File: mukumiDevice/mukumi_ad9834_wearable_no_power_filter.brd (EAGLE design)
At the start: 54 x 90 mm, 131 parts, among them IC1A1 1k, IC1A1,1 1k, IC1A3'1 560, IC1B1 1k, IC1B2 1k, IC1B6,1 2k, IC2A1,1 5.1k, IC2A3 20k, IC2A3,2 20k, IC2A4 5.1k, IC2B1 20k, IC2B2 5.1k, IC2B3 20k, IC2B6,1 5.1k, IC3A2 56, IC3B1 56, IC4 TL072D, IC4A1 560, IC4A2,2 560, IC4B1 62a, IC4B2 560, IC4B6,1 560a, IC4B6,10 560a, IC4B6,11 560a, IC4B6,12 560a, IC4B6,13 560a, IC4B6,2 560a, IC4B6,3 560a, IC4B6,4 560a, IC4B6,5 560a, IC4B6,6 560a, IC4B6,7 560a, IC4B6,8 560a, IC4B6,9 560a, U1 AD9834, U2 AD9834

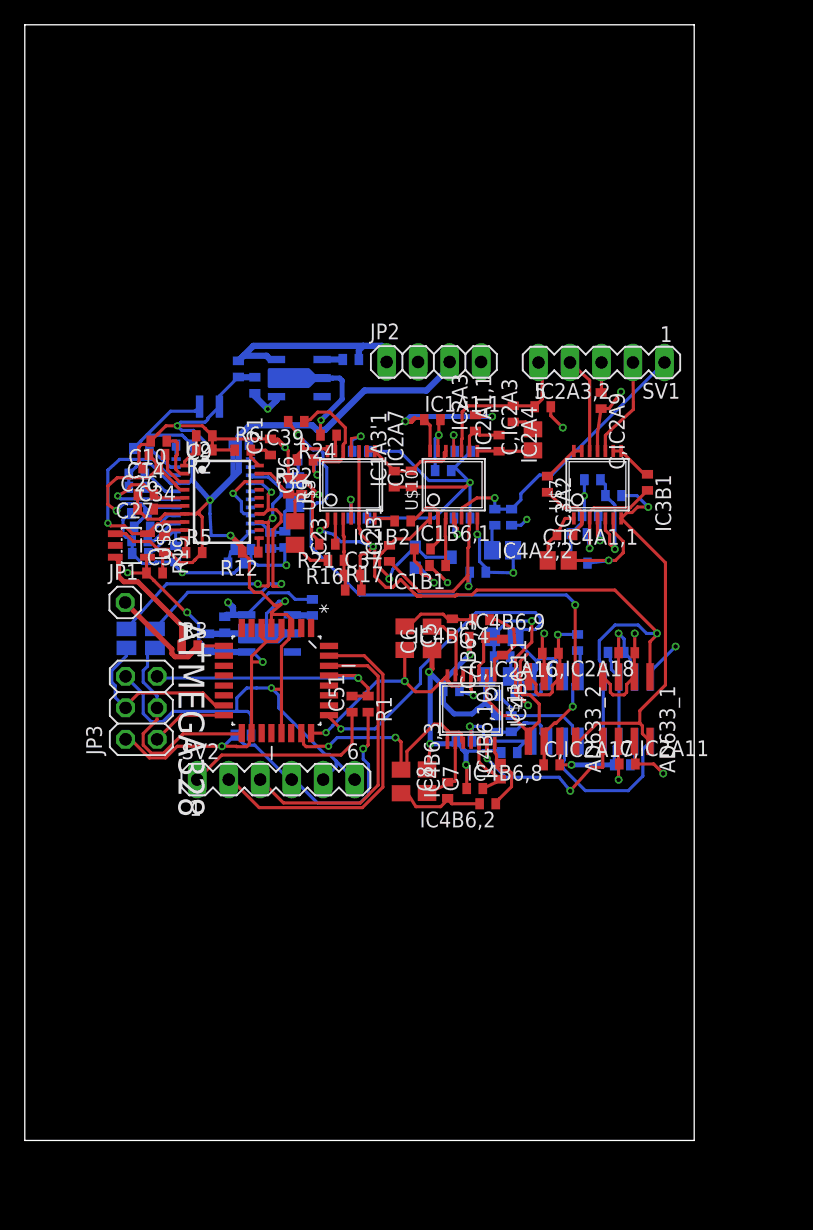
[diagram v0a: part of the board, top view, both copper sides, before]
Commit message: bNAMEの整理と部品名の整理
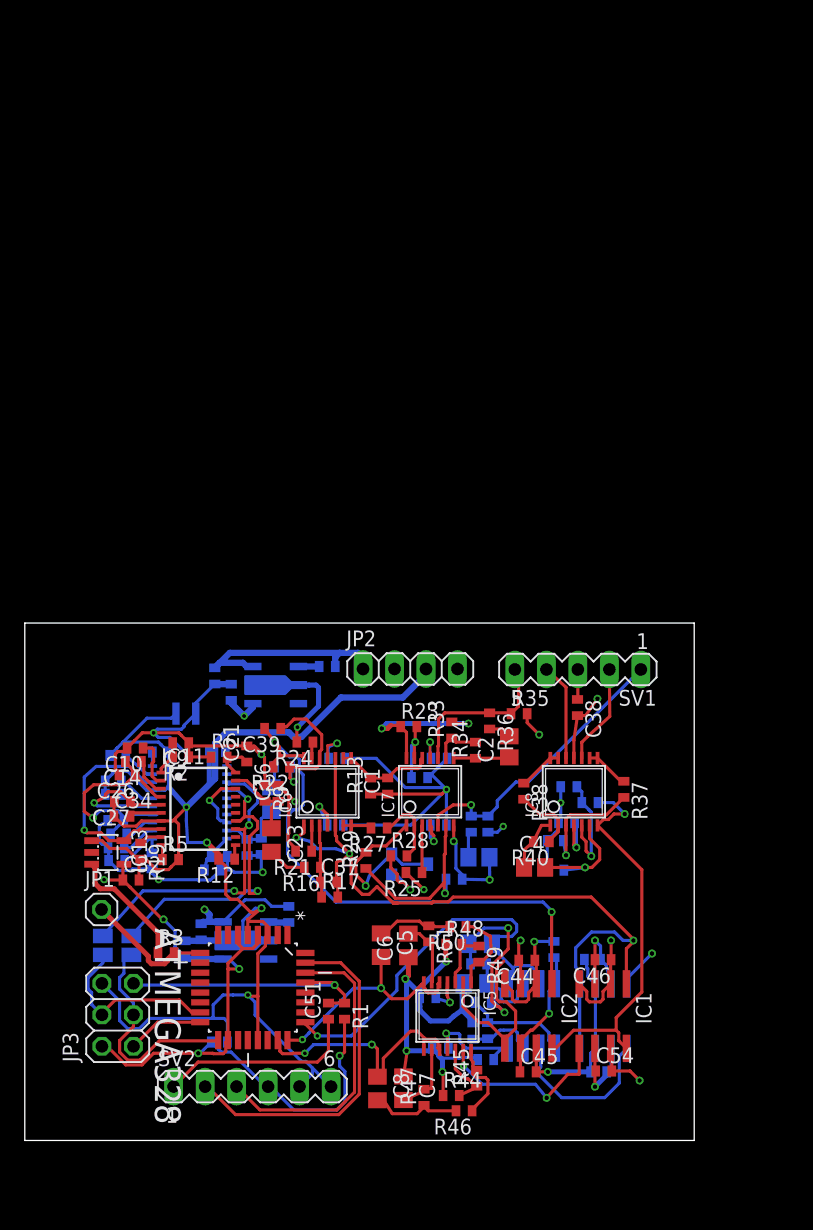
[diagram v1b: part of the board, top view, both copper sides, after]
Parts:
- removed AD633_1, AD633_2, AD633_3: AD835, linear:SO08
- removed C,IC2A1, C,IC2A10, C,IC2A11, C,IC2A12, C,IC2A13, C,IC2A14, C,IC2A15, C,IC2A16, C,IC2A17, C,IC2A18, C,IC2A2, C,IC2A4, C,IC2A5, C,IC2A6, C,IC2A7, C,IC2A8, C,IC2A9: 0.1u, rcl:C0402
- removed C,IC2A3, CIC2B1: 4.7u, rcl:C2012
- removed C,IC4A1,1: 0.47u, rcl:C2012
- removed IC1A1, IC1A1,1, IC1B1, IC1B2: 1k, rcl:R0402
- removed IC1A3'1, IC4A1, IC4A2,2, IC4B2: 560, rcl:R0402
- removed IC1B6,1: 2k, rcl:R0402
- removed IC2A1,1, IC2A4, IC2B2, IC2B6,1: 5.1k, rcl:R0402
- removed IC2A3, IC2A3,2, IC2B1, IC2B3: 20k, rcl:R0402
- removed IC3A2, IC3B1: 56, rcl:R0402
- removed IC4B1: 62a, rcl:R0402
- removed IC4B6,1, IC4B6,10, IC4B6,11, IC4B6,12, IC4B6,13, IC4B6,2, IC4B6,3, IC4B6,4, IC4B6,5, IC4B6,6, IC4B6,7, IC4B6,8, IC4B6,9: 560a, rcl:R0402
- removed L2: CB2016, inductor-yuden:CB2016
- removed U$1, U$2: NJM2884, torex:SOT89-5
- removed U$10, U$11, U$3, U$7: NJM074V, linear:TSSOP14
- removed U$4: PVZ3A, pvz3:PVZ3A
- removed U$8: SIT8002B, memsOsc:SOT25
- removed U1, U2: AD9834, ad9834:TSSOP20
- added C1, C11, C12, C22, C38, C41, C42, C43, C44, C45, C46, C48, C49, C50, C53, C54, C55: 0.1u, rcl:C0402
- added C2, C3: 4.7u, rcl:C2012
- added C4: 0.47u, rcl:C2012
- added IC1, IC2, IC3: AD835, linear:SO08
- added IC10, IC9: NJM2884, torex:SOT89-5
- added IC11, IC12: AD9834, ad9834:TSSOP20
- added IC13: SIT8002B, memsOsc:SOT25
- added IC5, IC6, IC7, IC8: NJM074V, linear:TSSOP14
- added L1: CB2016, inductor-yuden:CB2016
- added R13, R39, R40, R41: 560, rcl:R0402
- added R20, R23, R25, R27: 1k, rcl:R0402
- added R28: 2k, rcl:R0402
- added R29, R32, R33, R35: 20k, rcl:R0402
- added R30, R31, R34, R36: 5.1k, rcl:R0402
- added R37, R38: 56, rcl:R0402
- added R42: 62a, rcl:R0402
- added R43, R44, R45, R46, R47, R48, R49, R50, R51, R52, R53, R54, R55: 560a, rcl:R0402
- added VR1: PVZ3A, pvz3:PVZ3A
- moved C13 24.8 mm to (7.13, 29.0)
- moved C16 24.8 mm to (20.4, 28.0)
- moved C17 24.8 mm to (15.1, 21.8)
- moved C27 24.8 mm to (7.87, 27.3)
- moved C28 24.8 mm to (7.14, 27.9)
- moved C32 24.8 mm to (8.56, 21.0)
- moved C35 24.8 mm to (7.37, 23.6)
- moved C52 24.8 mm to (15.7, 7.93)
- moved R14 24.8 mm to (15.5, 31.4)
- moved R4 24.8 mm to (7.50, 31.1)
- moved ATMEGA328 24.8 mm to (18.4, 12.3)
- moved C18 24.8 mm to (14.2, 16.8)
- moved C19 24.8 mm to (12.9, 15.5)
- moved C20 24.8 mm to (19.1, 23.7)
- moved C23 24.8 mm to (19.9, 24.2)
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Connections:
- net +5V: now also C11.1, C22.1, C41.1, C43.1, C45.1, C48.1, C50.1, C54.1, IC1.6, IC2.6, IC3.6, IC5.4, IC6.4, IC7.4, IC8.4; no longer AD633_1.6, AD633_2.6, AD633_3.6, C,IC2A1.1, C,IC2A11.1, C,IC2A15.1, C,IC2A17.1, C,IC2A2.1, C,IC2A4.1, C,IC2A5.1, C,IC2A6.1, U$10.4, U$11.4, U$3.4, U$7.4
- net +BATTERY: now also IC10.5, IC9.5; no longer U$1.5, U$2.5
- net -5V: now also C12.2, C38.2, C42.2, C44.2, C46.2, C49.2, C53.2, C55.2, IC1.3, IC2.3, IC3.3, IC5.11, IC6.11, IC7.11, IC8.11; no longer AD633_1.3, AD633_2.3, AD633_3.3, C,IC2A10.2, C,IC2A12.2, C,IC2A13.2, C,IC2A14.2, C,IC2A16.2, C,IC2A18.2, C,IC2A8.2, C,IC2A9.2, U$10.11, U$11.11, U$3.11, U$7.11
- net 3.3V_DDS: now also IC10.4, IC11.4, IC12.4; no longer U$2.4, U1.4, U2.4
- net 3.3V_MC: now also IC11.5, IC12.5, IC13.4, IC9.4; no longer U$1.4, U$8.4, U1.5, U2.5
- net A1: now also C3.1, IC7.7, R30.1; no longer CIC2B1.1, IC2B6,1.1, U$10.7
- net AGND: now also C1.1, C11.2, C12.1, C22.2, C38.1, C41.2, C42.1, C43.2, C44.1, C45.2, C46.1, C48.2, C49.1, C50.2, C53.1, C54.2, C55.1, IC1.2, IC1.4, IC1.7, IC10.2, IC11.18, IC12.18, IC2.2, IC2.4, IC2.7, IC3.2, IC3.4, IC3.7, L1.1, R13.1, R20.1, R25.2, R32.2, R35.2, R39.2, R41.1, R42.1, R44.1, R48.1, R52.1; no longer AD633_1.2, AD633_1.4, AD633_1.7, AD633_2.2, AD633_2.4, AD633_2.7, AD633_3.2, AD633_3.4, AD633_3.7, C,IC2A1.2, C,IC2A10.1, C,IC2A11.2, C,IC2A12.1, C,IC2A13.1, C,IC2A14.1, C,IC2A15.2, C,IC2A16.1, C,IC2A17.2, C,IC2A18.1, C,IC2A2.2, C,IC2A4.2, C,IC2A5.2, C,IC2A6.2, C,IC2A7.1, C,IC2A8.1, C,IC2A9.1, IC1A1.1, IC1A3'1.1, IC1B1.2, IC2A3,2.2, IC2B3.2, IC4A1.2, IC4B1.1, IC4B2.1, IC4B6,12.1, IC4B6,8.1, IC4B6,9.1, L2.1, U$2.2, U1.18, U2.18
- net COS: now also IC2.1, IC6.14; no longer AD633_2.1, U$3.14
- net DDS_OUT1: now also IC11.19; no longer U2.19
- net DDS_OUT1B: now also IC11.20; no longer U2.20
- net DDS_OUT2: now also IC12.19; no longer U1.19
- net DDS_OUT2B: now also IC12.20; no longer U1.20
- net DENKYOKU1: now also IC8.12; no longer U$7.12
- net DENKYOKU2: now also IC8.10; no longer U$7.10
- net FSYNC1: now also IC11.15; no longer U2.15
- net FSYNC2: now also IC12.15; no longer U1.15
- net GND: now also IC11.7, IC12.7, IC13.1, IC9.2, L1.2; no longer L2.2, U$1.2, U$8.1, U1.7, U2.7
- net I1: now also IC7.10, R35.1, R36.1; no longer IC2A3,2.1, IC2A4.1, U$10.10
- net I2: now also IC7.5, R31.1, R32.1; no longer IC2B2.1, IC2B3.1, U$10.5
- net N$1: now also IC6.2; no longer U$3.2
- net N$10: now also IC12.6; no longer U1.6
- net N$11: now also IC13.3; no longer U$8.3
- net N$12: now also R53.2, R54.1; no longer IC4B6,13.2, IC4B6,6.1
- net N$13: now also IC9.1; no longer U$1.1
- net N$14: now also IC10.1; no longer U$2.1
- net N$17: now also IC5.12, R44.2, R45.1; no longer IC4B6,10.1, IC4B6,8.2, U$11.12
- net N$19: now also R55.2; no longer IC4B6,7.2
- net N$2: now also IC5.6, R51.2; no longer IC4B6,5.2, U$11.6
- net N$22: now also IC12.1; no longer U1.1
- net N$25: now also IC11.6; no longer U2.6
- net N$26: now also IC7.13, R20.2, R23.2; no longer IC1A1,1.2, IC1A1.2, U$10.13
- net N$27: now also IC11.9; no longer U2.9
- net N$28: now also IC12.9; no longer U1.9
- net N$29: now also IC12.11; no longer U1.11
- net N$3: now also IC5.9, R47.2; no longer IC4B6,3.2, U$11.9
- net N$30: now also IC12.10; no longer U1.10
- net N$33: now also IC7.14, R23.1, R33.2; no longer IC1A1,1.1, IC2A3.2, U$10.14
- net N$38: now also IC12.12; no longer U1.12
- net N$39: now also IC6.13; no longer U$3.13
- net N$4: now also R50.2, R51.1; no longer IC4B6,4.2, IC4B6,5.1
- net N$40: now also IC7.9, R33.1, R34.2; no longer IC2A1,1.2, IC2A3.1, U$10.9
- net N$41: now also C2.2, R36.2; no longer C,IC2A3.2, IC2A4.2
- net N$43: now also IC5.3, R48.2, R49.1; no longer IC4B6,11.1, IC4B6,9.2, U$11.3
- net N$44: now also IC7.6, R29.1, R30.2; no longer IC2B1.1, IC2B6,1.2, U$10.6
- net N$45: now also IC2.5, IC5.2; no longer AD633_2.5, U$11.2
- net N$46: now also C3.2, R31.2; no longer CIC2B1.2, IC2B2.2
- net N$47: now also IC7.2, R27.1, R28.2; no longer IC1B2.1, IC1B6,1.2, U$10.2
- net N$48: now also IC7.1, R29.2, VR1.P$1, VR1.P$3; no longer IC2B1.2, U$10.1, U$4.P$1, U$4.P$3
- net N$49: now also R28.1, VR1.P$2; no longer IC1B6,1.1, U$4.P$2
- net N$5: now also IC1.5, IC5.13; no longer AD633_1.5, U$11.13
- net N$50: now also IC8.13, IC8.14, R38.1; no longer IC3A2.1, U$7.13, U$7.14
- net N$51: now also IC8.8, IC8.9, R37.1; no longer IC3B1.1, U$7.8, U$7.9
- net N$52: now also IC8.3, R37.2, R39.1; no longer IC3B1.2, IC4A1.1, U$7.3
- net N$53: now also IC8.2, R38.2, R40.1; no longer IC3A2.2, IC4A2,2.1, U$7.2
- net N$54: now also C4.1, IC8.1, R40.2; no longer C,IC4A1,1.1, IC4A2,2.2, U$7.1
- net N$55: now also C4.2, IC8.6, R41.2; no longer C,IC4A1,1.2, IC4B2.2, U$7.6
- net N$56: now also C2.1, IC7.8, R34.1; no longer C,IC2A3.1, IC2A1,1.1, U$10.8
- net N$57: now also IC7.3, R25.1; no longer IC1B1.1, U$10.3
- net N$58: now also IC8.5, R42.2, R43.1; no longer IC4B1.2, IC4B6,1.1, U$7.5
- net N$59: now also IC5.14, R45.2, R46.1; no longer IC4B6,10.2, IC4B6,2.1, U$11.14
- net N$6: now also R46.2, R47.1; no longer IC4B6,2.2, IC4B6,3.1
- net N$60: now also IC5.1, R49.2, R50.1; no longer IC4B6,11.2, IC4B6,4.1, U$11.1
- net N$61: now also C1.2, IC6.8, IC6.9, IC7.12, R13.2; no longer C,IC2A7.2, IC1A3'1.2, U$10.12, U$3.8, U$3.9
- net N$62: now also IC6.6, IC6.7, R27.2; no longer IC1B2.2, U$3.6, U$3.7
- net N$63: now also R54.2, R55.1; no longer IC4B6,6.2, IC4B6,7.1
- net N$66: now also IC11.11; no longer U2.11
- net N$67: now also IC11.1; no longer U2.1
- net N$68: now also IC3.5; no longer AD633_3.5
- net N$70: now also R52.2, R53.1; no longer IC4B6,12.2, IC4B6,13.1
- net N$74: now also IC11.10; no longer U2.10
- net N$75: now also IC12.2; no longer U1.2
- net N$77: now also IC12.3; no longer U1.3
- net N$78: now also IC6.3; no longer U$3.3
- net N$79: now also IC11.3; no longer U2.3
- net N$8: now also IC11.8, IC12.8, IC13.5; no longer U$8.5, U1.8, U2.8
- net N$9: now also IC11.2; no longer U2.2
- net N$91: now also IC6.12; no longer U$3.12
- net SCLK: now also IC11.14, IC12.14; no longer U1.14, U2.14
- net SDATA: now also IC11.13, IC12.13; no longer U1.13, U2.13
- net SIG: now also IC1.8, IC2.8, IC8.7, R43.2; no longer AD633_1.8, AD633_2.8, IC4B6,1.2, U$7.7
- net SIG*COS: now also IC5.5, IC5.7; no longer U$11.5, U$11.7
- net SIG*SIN: now also IC5.10, IC5.8; no longer U$11.10, U$11.8
- net SIN: now also IC1.1, IC3.1, IC3.8, IC6.1, IC6.10, IC6.5; no longer AD633_1.1, AD633_3.1, AD633_3.8, U$3.1, U$3.10, U$3.5
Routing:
- net +5V: track 108.5 -> 110.7 mm
- net N$70: track 6.07 -> 5.47 mm
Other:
- board size 54 x 90 mm -> 54 x 41.7 mm
- board text added: "VR1"
